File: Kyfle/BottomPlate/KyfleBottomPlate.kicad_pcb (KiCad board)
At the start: 2 copper layers, 164 x 146.2 mm, 52 parts, among them SW2 KEY_SWITCH, SW2 PRO MICRO

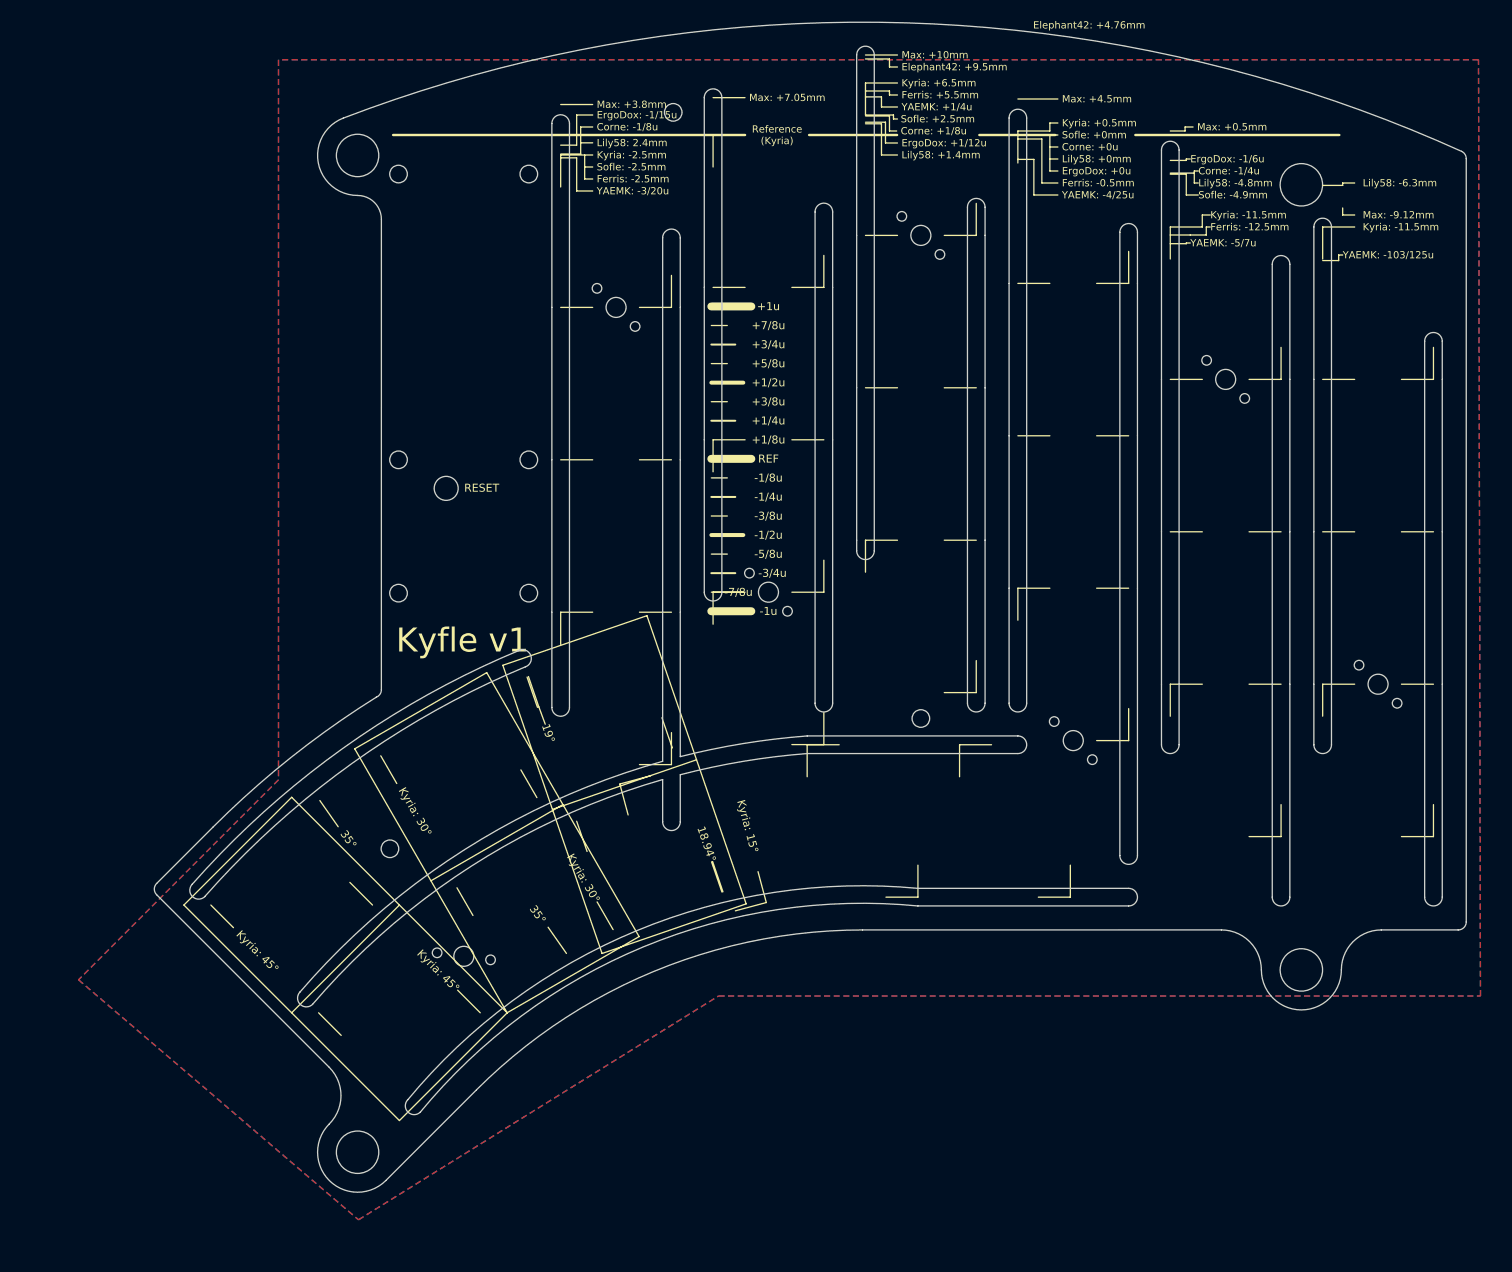
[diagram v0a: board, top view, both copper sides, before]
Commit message: Touch ups and small works
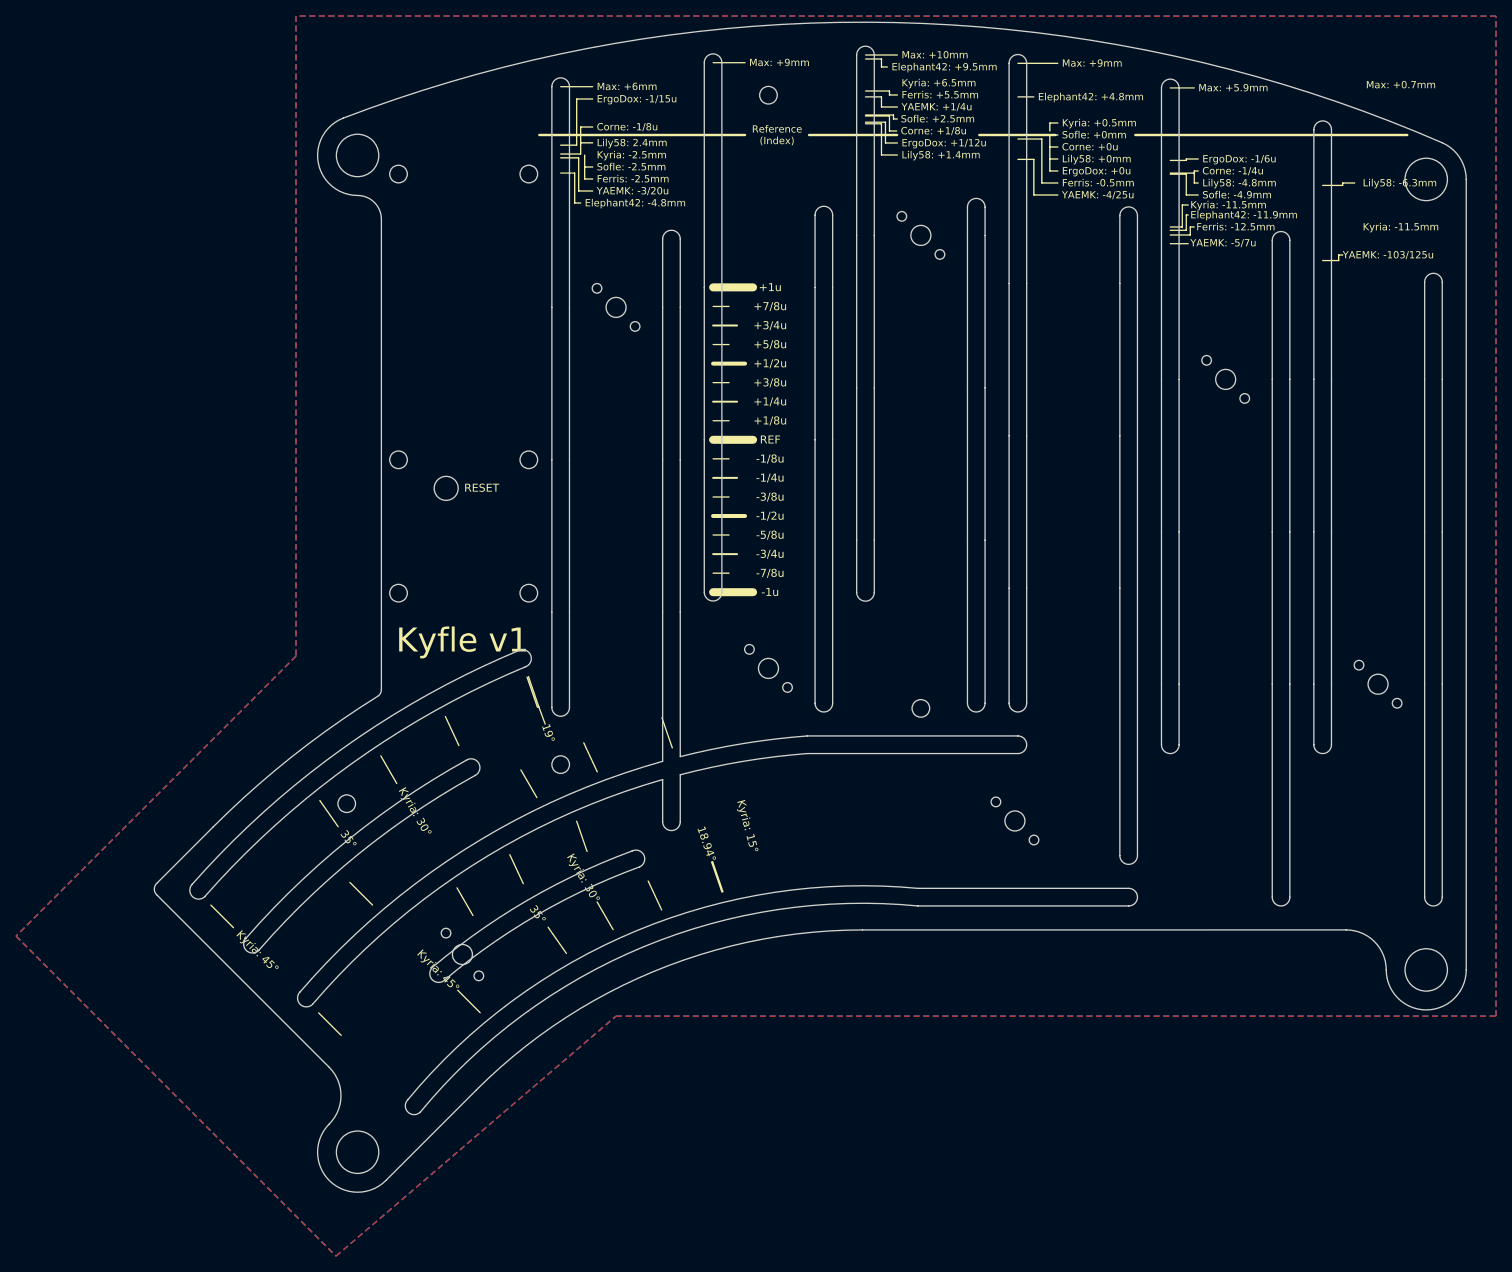
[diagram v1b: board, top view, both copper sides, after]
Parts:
- removed the REF** at (216.6, 38.6)
- removed the REF** at (216.6, 136.7)
- added REF**: MountingHole_2.2mm_M2_ISO14580, Kyfle Footprints:M5_with_washer_and_board, F.Cu at (237.2, 136.7)
- added REF**: MountingHole_2.2mm_M2_ISO14580, Kyfle Footprints:M5_with_washer, F.Cu at (232.2, 37.9)
- added Ref**: Val**, Kyfle Footprints:M2_with_washer, F.Cu at (124.0, 111.1)
- added SW2: KEY_SWITCH, Kyfle Footprints:CherryMX_Kyfle_v1_BottomPlate_2u, F.Cu at (123.1, 117.2)
- moved Spacer 25.2 mm to (118.5, 65.9), turned to 180 degrees
- moved SW2 12.4 mm to (180.8, 118.1)
- moved TH3 12.1 mm to (150.0, 27.4)
- moved SW2 9.52 mm to (150.0, 99.0)
- moved TH7 7.81 mm to (97.3, 116.0)
- moved TH7 1.26 mm to (169.1, 104.0)
- moved SW2 0.29 mm to (111.7, 134.8), turned to 352.5 degrees
- turned SW2 to 225 degrees
- turned SW2 to 210 degrees
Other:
- board size 164 x 146.2 mm -> 164 x 146.3 mm
- board text added: "Elephant42: +4.8mm"
- board text added: "Elephant42: -11.9mm"
- board text added: "Elephant42: -4.8mm"
- board text added: "Max: +0.7mm"
- board text added: "Max: +5.9mm"
- board text added: "Max: +6mm"
- board text added: "Max: +9mm"
- board text added: "Reference (Index)"
- board text removed: "Elephant42: +4.76mm"
- board text removed: "Max: +0.5mm"
- board text removed: "Max: +4.5mm"
- board text removed: "Max: -9.12mm"
